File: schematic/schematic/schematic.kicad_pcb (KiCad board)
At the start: 2 copper layers, 4 parts, among them J1 Conn_01x05, U1 74AHCT125

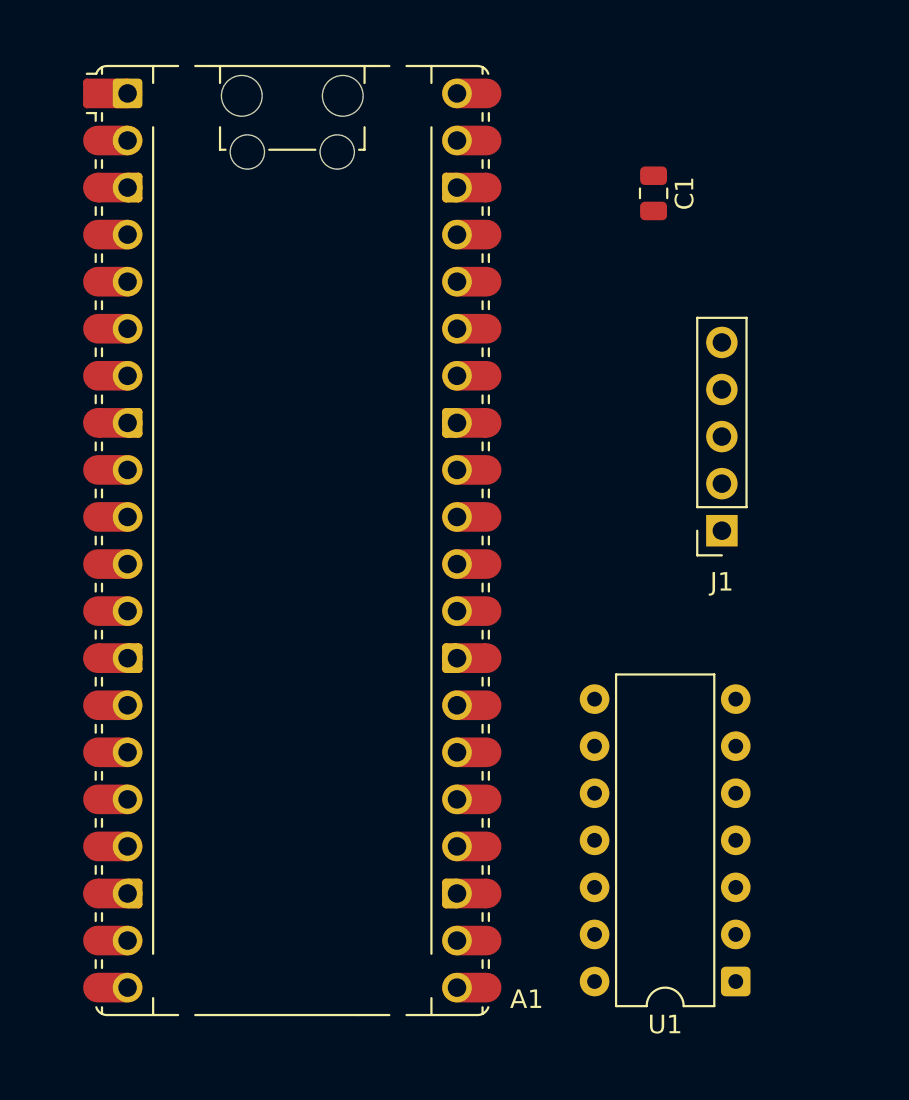
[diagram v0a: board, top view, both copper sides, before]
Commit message: finished the PCB and added the images
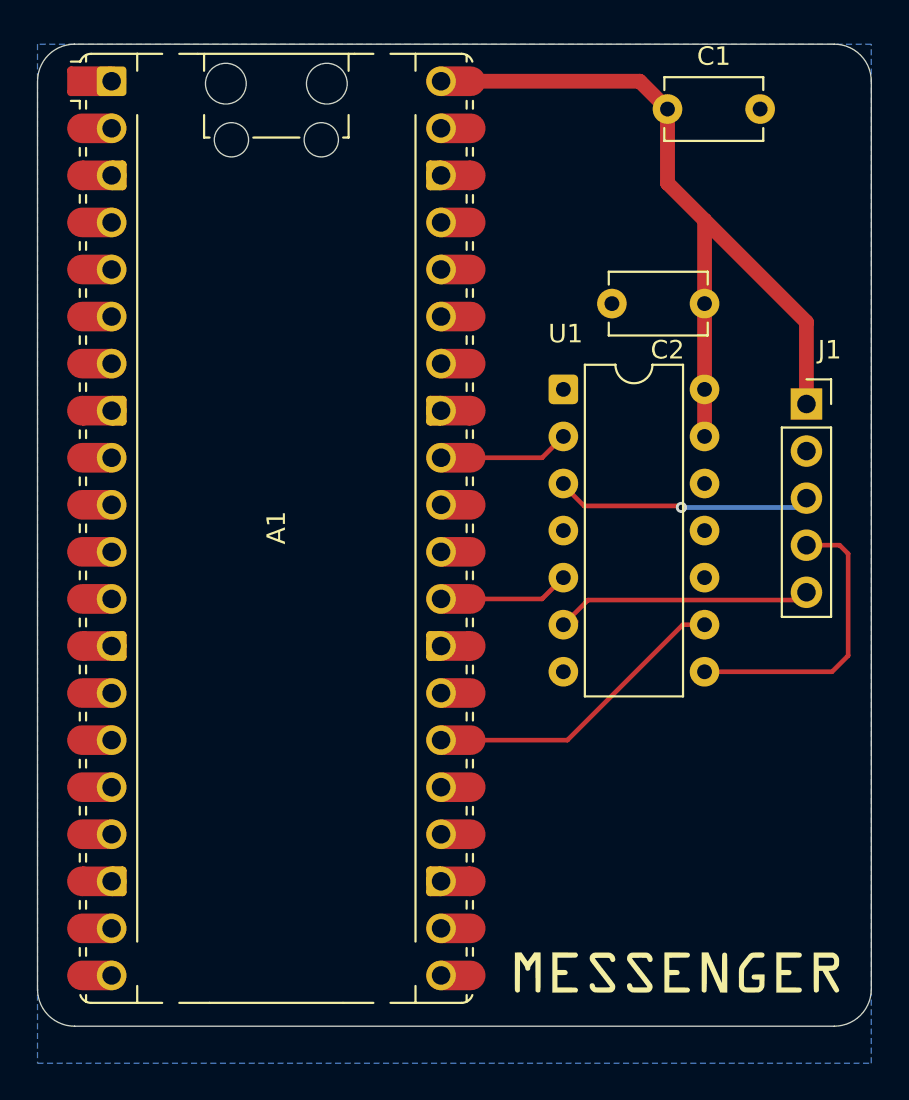
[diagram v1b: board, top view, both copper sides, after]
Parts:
- added C2: nF100, Capacitor_THT:C_Disc_D5.1mm_W3.2mm_P5.00mm, F.Cu at (156.0, 89.0)
- added G***: LOGO, LOGO, F.Cu at (154.5, 122.8)
- C1: value C -> uF10; footprint Capacitor_SMD:C_0805_2012Metric -> Capacitor_THT:C_Disc_D5.1mm_W3.2mm_P5.00mm
- moved U1 33.3 mm to (148.4, 93.6), turned to 0 degrees
- moved J1 8.22 mm to (161.5, 94.4), turned to 0 degrees
- moved C1 4.61 mm to (154.0, 78.5), turned to 0 degrees
- moved A1 1.08 mm to (132.9, 101.1)
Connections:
- A1 pad 21: /PICO_DIN -> unconnected-(A1-GPIO16-Pad21)_1
- A1 pad 22: /PICO_CLK -> unconnected-(A1-GPIO17-Pad22)_1
- A1 pad 24: /PICO_CS -> unconnected-(A1-GPIO18-Pad24)_1
- A1 pad 26: unconnected-(A1-GPIO20-Pad26) -> /PICO_CS
- A1 pad 29: unconnected-(A1-GPIO22-Pad29) -> /PICO_CLK
- A1 pad 32: unconnected-(A1-GPIO27_ADC1-Pad32) -> /PICO_DIN
- U1 pad 11: (no net) -> unconnected-(U1-Pad11)
- U1 pad 12: (no net) -> GND
- U1 pad 13: (no net) -> +5V
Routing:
- net +5V: track 0.00 -> 43.9 mm
- net /PICO_CS: track 0.00 -> 16.8 mm
- net /MTX_CS: track 0.00 -> 16.1 mm
- net /MTX_CLK: track 0.00 -> 14.8 mm
- net /MTX_DIN: track 0.00 -> 14.3 mm, vias 0 -> 1
- net /PICO_DIN: track 0.00 -> 7.08 mm
- net /PICO_CLK: track 0.00 -> 7.08 mm
- added copper zone on B.Cu, net GND
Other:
- board outline added: 45 x 53 mm
